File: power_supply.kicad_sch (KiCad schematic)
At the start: 18 parts, among them J1 Разъём к автомобилю 2x16 (32 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, U6 MC78M05CDTG, U7 AMS1117-3.3

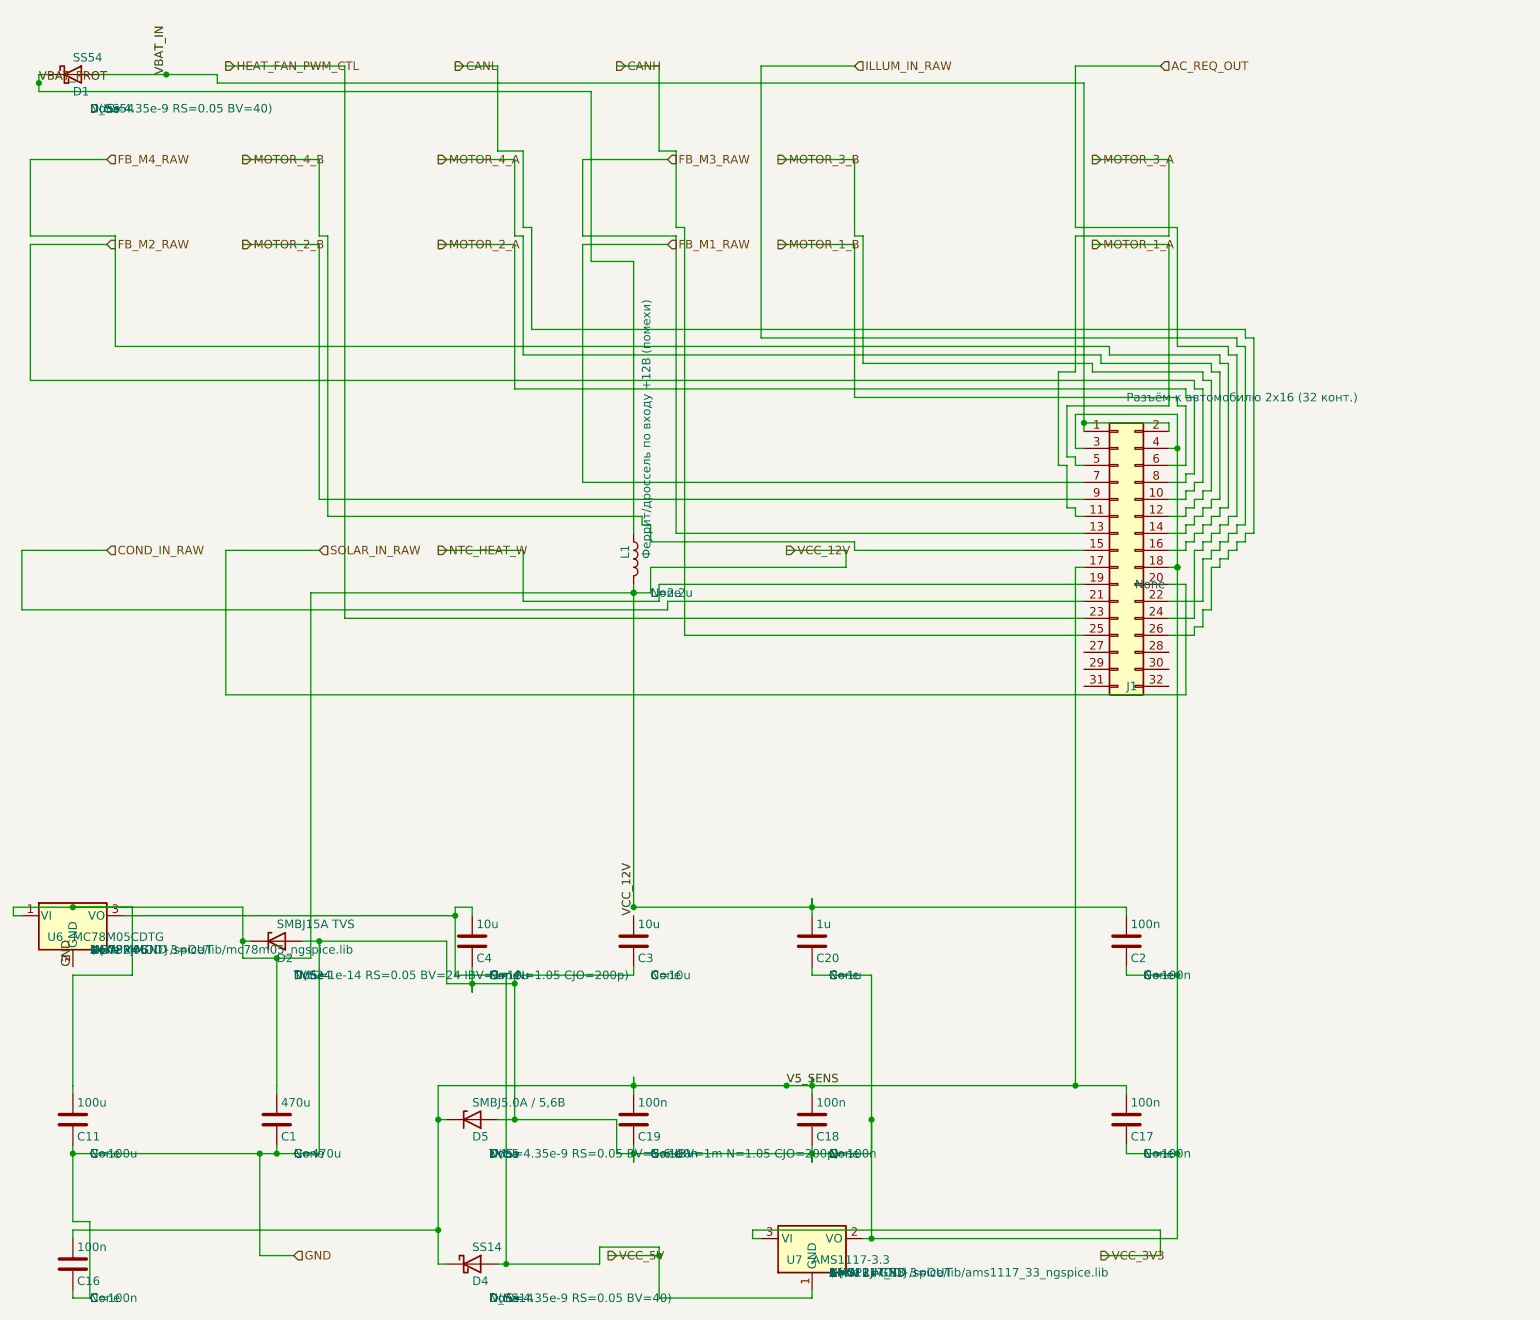
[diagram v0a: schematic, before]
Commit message: multiInstance path fix
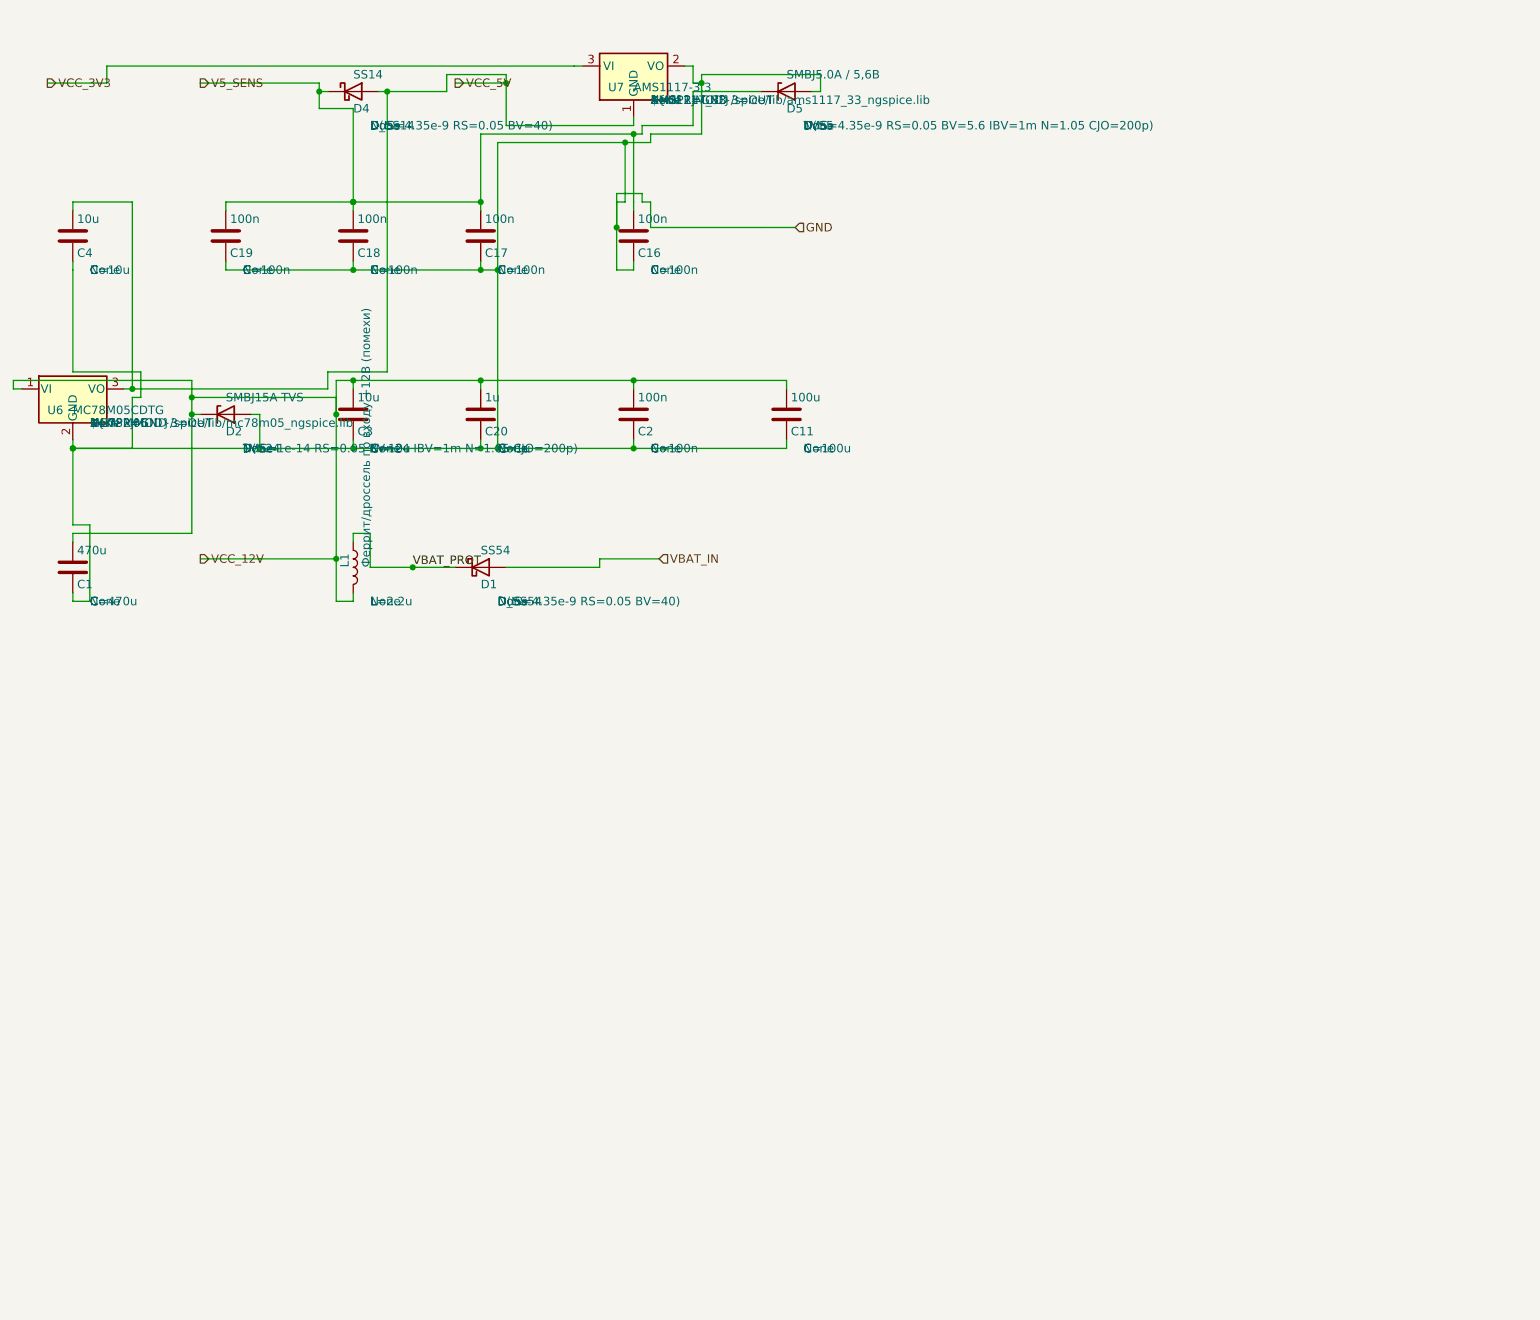
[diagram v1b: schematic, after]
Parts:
- removed J1: Разъём к автомобилю 2x16 (32 конт.), symbol Connector_Generic:Conn_02x16_Odd_Even

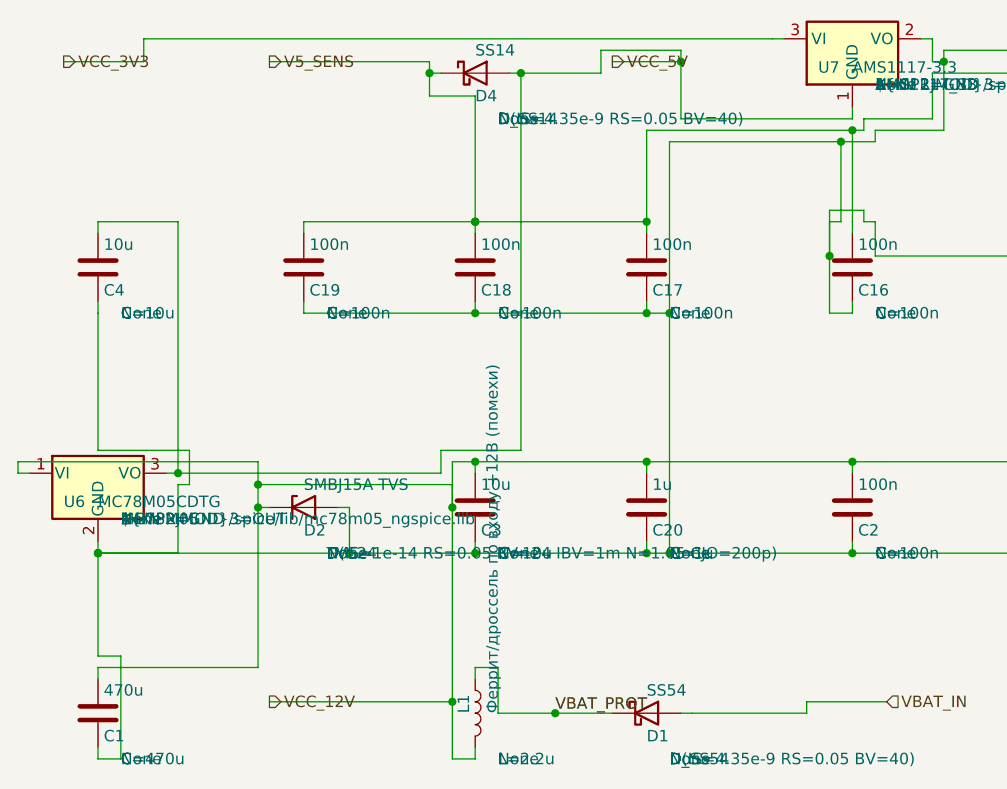
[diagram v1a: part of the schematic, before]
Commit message: fix
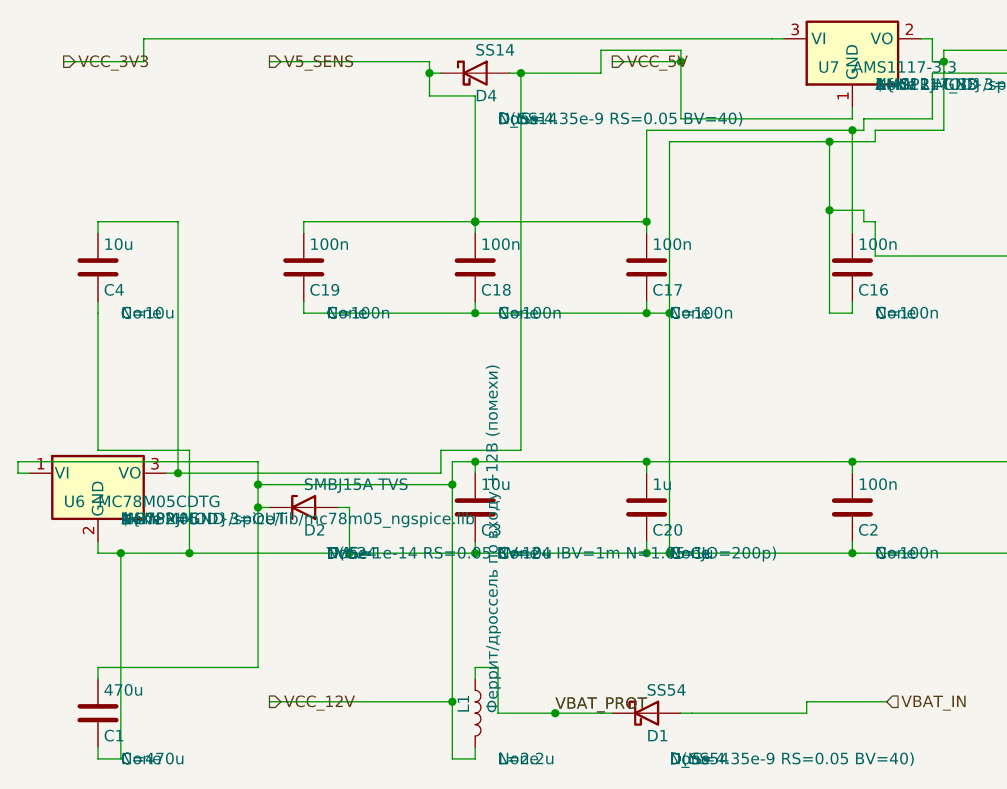
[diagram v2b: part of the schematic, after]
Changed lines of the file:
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@@
 				(instances
 			(project "climate_control_niva_travel"
-				(path "/a20a8d43-2e18-4318-8ef3-7f434a470dab/595b8d41-035e-473d-8fdc-63eaba4c2891"(reference "C0201") (unit 1) )
+				(path "/c1309681-e2dd-46a3-91f6-d828d5f4c0f8"(reference "C1") (unit 1) )
+				(path "/aece091b-8e26-4b21-9786-1b0efc647a51/aaf05096-9cf9-4019-8237-5c0c69cd71a7"(reference "C0201") (unit 1) )
 			)
 		)
@@
 				(instances
 			(project "climate_control_niva_travel"
-				(path "/a20a8d43-2e18-4318-8ef3-7f434a470dab/595b8d41-035e-473d-8fdc-63eaba4c2891"(reference "C0211") (unit 1) )
+				(path "/c1309681-e2dd-46a3-91f6-d828d5f4c0f8"(reference "C11") (unit 1) )
+				(path "/aece091b-8e26-4b21-9786-1b0efc647a51/aaf05096-9cf9-4019-8237-5c0c69cd71a7"(reference "C0211") (unit 1) )
 			)
 		)
@@
 				(instances
 			(project "climate_control_niva_travel"
-				(path "/a20a8d43-2e18-4318-8ef3-7f434a470dab/595b8d41-035e-473d-8fdc-63eaba4c2891"(reference "C0216") (unit 1) )
+				(path "/c1309681-e2dd-46a3-91f6-d828d5f4c0f8"(reference "C16") (unit 1) )
+				(path "/aece091b-8e26-4b21-9786-1b0efc647a51/aaf05096-9cf9-4019-8237-5c0c69cd71a7"(reference "C0216") (unit 1) )
 			)
 		)
@@
 				(instances
 			(project "climate_control_niva_travel"
-				(path "/a20a8d43-2e18-4318-8ef3-7f434a470dab/595b8d41-035e-473d-8fdc-63eaba4c2891"(reference "C0217") (unit 1) )
+				(path "/c1309681-e2dd-46a3-91f6-d828d5f4c0f8"(reference "C17") (unit 1) )
+				(path "/aece091b-8e26-4b21-9786-1b0efc647a51/aaf05096-9cf9-4019-8237-5c0c69cd71a7"(reference "C0217") (unit 1) )
 			)
 		)
@@
 				(instances
 			(project "climate_control_niva_travel"
-				(path "/a20a8d43-2e18-4318-8ef3-7f434a470dab/595b8d41-035e-473d-8fdc-63eaba4c2891"(reference "C0218") (unit 1) )
+				(path "/c1309681-e2dd-46a3-91f6-d828d5f4c0f8"(reference "C18") (unit 1) )
+				(path "/aece091b-8e26-4b21-9786-1b0efc647a51/aaf05096-9cf9-4019-8237-5c0c69cd71a7"(reference "C0218") (unit 1) )
 			)
 		)
@@
 				(instances
 			(project "climate_control_niva_travel"
-				(path "/a20a8d43-2e18-4318-8ef3-7f434a470dab/595b8d41-035e-473d-8fdc-63eaba4c2891"(reference "C0219") (unit 1) )
+				(path "/c1309681-e2dd-46a3-91f6-d828d5f4c0f8"(reference "C19") (unit 1) )
+				(path "/aece091b-8e26-4b21-9786-1b0efc647a51/aaf05096-9cf9-4019-8237-5c0c69cd71a7"(reference "C0219") (unit 1) )
 			)
 		)
@@
 				(instances
 			(project "climate_control_niva_travel"
-				(path "/a20a8d43-2e18-4318-8ef3-7f434a470dab/595b8d41-035e-473d-8fdc-63eaba4c2891"(reference "C0202") (unit 1) )
+				(path "/c1309681-e2dd-46a3-91f6-d828d5f4c0f8"(reference "C2") (unit 1) )
+				(path "/aece091b-8e26-4b21-9786-1b0efc647a51/aaf05096-9cf9-4019-8237-5c0c69cd71a7"(reference "C0202") (unit 1) )
 			)
 		)
@@
 				(instances
 			(project "climate_control_niva_travel"
-				(path "/a20a8d43-2e18-4318-8ef3-7f434a470dab/595b8d41-035e-473d-8fdc-63eaba4c2891"(reference "C0220") (unit 1) )
+				(path "/c1309681-e2dd-46a3-91f6-d828d5f4c0f8"(reference "C20") (unit 1) )
+				(path "/aece091b-8e26-4b21-9786-1b0efc647a51/aaf05096-9cf9-4019-8237-5c0c69cd71a7"(reference "C0220") (unit 1) )
 			)
 		)
@@
 				(instances
 			(project "climate_control_niva_travel"
-				(path "/a20a8d43-2e18-4318-8ef3-7f434a470dab/595b8d41-035e-473d-8fdc-63eaba4c2891"(reference "C0203") (unit 1) )
+				(path "/c1309681-e2dd-46a3-91f6-d828d5f4c0f8"(reference "C3") (unit 1) )
+				(path "/aece091b-8e26-4b21-9786-1b0efc647a51/aaf05096-9cf9-4019-8237-5c0c69cd71a7"(reference "C0203") (unit 1) )
 			)
 		)
@@
 				(instances
 			(project "climate_control_niva_travel"
-				(path "/a20a8d43-2e18-4318-8ef3-7f434a470dab/595b8d41-035e-473d-8fdc-63eaba4c2891"(reference "C0204") (unit 1) )
+				(path "/c1309681-e2dd-46a3-91f6-d828d5f4c0f8"(reference "C4") (unit 1) )
+				(path "/aece091b-8e26-4b21-9786-1b0efc647a51/aaf05096-9cf9-4019-8237-5c0c69cd71a7"(reference "C0204") (unit 1) )
 			)
 		)
@@
 				(instances
 			(project "climate_control_niva_travel"
-				(path "/a20a8d43-2e18-4318-8ef3-7f434a470dab/595b8d41-035e-473d-8fdc-63eaba4c2891"(reference "D0201") (unit 1) )
+				(path "/c1309681-e2dd-46a3-91f6-d828d5f4c0f8"(reference "D1") (unit 1) )
+				(path "/aece091b-8e26-4b21-9786-1b0efc647a51/aaf05096-9cf9-4019-8237-5c0c69cd71a7"(reference "D0201") (unit 1) )
 			)
 		)
@@
 				(instances
 			(project "climate_control_niva_travel"
-				(path "/a20a8d43-2e18-4318-8ef3-7f434a470dab/595b8d41-035e-473d-8fdc-63eaba4c2891"(reference "D0202") (unit 1) )
+				(path "/c1309681-e2dd-46a3-91f6-d828d5f4c0f8"(reference "D2") (unit 1) )
+				(path "/aece091b-8e26-4b21-9786-1b0efc647a51/aaf05096-9cf9-4019-8237-5c0c69cd71a7"(reference "D0202") (unit 1) )
 			)
 		)
@@
 				(instances
 			(project "climate_control_niva_travel"
-				(path "/a20a8d43-2e18-4318-8ef3-7f434a470dab/595b8d41-035e-473d-8fdc-63eaba4c2891"(reference "D0204") (unit 1) )
+				(path "/c1309681-e2dd-46a3-91f6-d828d5f4c0f8"(reference "D4") (unit 1) )
+				(path "/aece091b-8e26-4b21-9786-1b0efc647a51/aaf05096-9cf9-4019-8237-5c0c69cd71a7"(reference "D0204") (unit 1) )
 			)
 		)
@@
 				(instances
 			(project "climate_control_niva_travel"
-				(path "/a20a8d43-2e18-4318-8ef3-7f434a470dab/595b8d41-035e-473d-8fdc-63eaba4c2891"(reference "D0205") (unit 1) )
+				(path "/c1309681-e2dd-46a3-91f6-d828d5f4c0f8"(reference "D5") (unit 1) )
+				(path "/aece091b-8e26-4b21-9786-1b0efc647a51/aaf05096-9cf9-4019-8237-5c0c69cd71a7"(reference "D0205") (unit 1) )
 			)
 		)
@@
 				(instances
 			(project "climate_control_niva_travel"
-				(path "/a20a8d43-2e18-4318-8ef3-7f434a470dab/595b8d41-035e-473d-8fdc-63eaba4c2891"(reference "L0201") (unit 1) )
+				(path "/c1309681-e2dd-46a3-91f6-d828d5f4c0f8"(reference "L1") (unit 1) )
+				(path "/aece091b-8e26-4b21-9786-1b0efc647a51/aaf05096-9cf9-4019-8237-5c0c69cd71a7"(reference "L0201") (unit 1) )
 			)
 		)
@@
 				(instances
 			(project "climate_control_niva_travel"
-				(path "/a20a8d43-2e18-4318-8ef3-7f434a470dab/595b8d41-035e-473d-8fdc-63eaba4c2891"(reference "U0206") (unit 1) )
+				(path "/c1309681-e2dd-46a3-91f6-d828d5f4c0f8"(reference "U6") (unit 1) )
+				(path "/aece091b-8e26-4b21-9786-1b0efc647a51/aaf05096-9cf9-4019-8237-5c0c69cd71a7"(reference "U0206") (unit 1) )
 			)
 		)
@@
 				(instances
 			(project "climate_control_niva_travel"
-				(path "/a20a8d43-2e18-4318-8ef3-7f434a470dab/595b8d41-035e-473d-8fdc-63eaba4c2891"(reference "U0207") (unit 1) )
+				(path "/c1309681-e2dd-46a3-91f6-d828d5f4c0f8"(reference "U7") (unit 1) )
+				(path "/aece091b-8e26-4b21-9786-1b0efc647a51/aaf05096-9cf9-4019-8237-5c0c69cd71a7"(reference "U0207") (unit 1) )
 			)
 		)
@@
 	(wire
 		(pts
-			(xy 50.8 53.34) (xy 50.8 55.88)
-		)
-		(stroke
-			(width 0)
-			(type default)
-		)
-	)
-	(wire
-		(pts
 			(xy 11.43 74.93) (xy 11.43 73.66)
 		)
@@
 	(wire
 		(pts
-			(xy 13.97 83.82) (xy 13.97 72.39)
-		)
-		(stroke
-			(width 0)
-			(type default)
-		)
-	)
-	(wire
-		(pts
-			(xy 13.97 72.39) (xy 11.43 72.39)
-		)
-		(stroke
-			(width 0)
-			(type default)
-		)
-	)
-	(wire
-		(pts
-			(xy 11.43 72.39) (xy 11.43 60.96)
+			(xy 13.97 83.82) (xy 13.97 60.96)
 		)
 		(stroke
@@
 	(wire
 		(pts
-			(xy 21.59 49.53) (xy 21.59 53.34)
-		)
-		(stroke
-			(width 0)
-			(type default)
-		)
-	)
-	(wire
-		(pts
-			(xy 21.59 53.34) (xy 20.32 53.34)
-		)
-		(stroke
-			(width 0)
-			(type default)
-		)
-	)
-	(wire
-		(pts
-			(xy 20.32 53.34) (xy 20.32 60.96)
-		)
-		(stroke
-			(width 0)
-			(type default)
-		)
-	)
-	(wire
-		(pts
-			(xy 20.32 60.96) (xy 11.43 60.96)
+			(xy 21.59 49.53) (xy 21.59 60.96)
 		)
 		(stroke
@@
 	(wire
 		(pts
-			(xy 92.71 34.29) (xy 92.71 24.13)
-		)
-		(stroke
-			(width 0)
-			(type default)
-		)
-	)
-	(wire
-		(pts
-			(xy 92.71 24.13) (xy 93.98 24.13)
-		)
-		(stroke
-			(width 0)
-			(type default)
-		)
-	)
-	(wire
-		(pts
-			(xy 93.98 24.13) (xy 93.98 15.24)
+			(xy 92.71 34.29) (xy 92.71 15.24)
 		)
 		(stroke
@@
 		)
 	)
-	(wire
-		(pts
-			(xy 92.71 22.86) (xy 92.71 27.94)
-		)
-		(stroke
-			(width 0)
-			(type default)
-		)
-	)
 	(junction
 		(at 53.34 50.8)
@@
 	)
 	(junction
-		(at 50.8 55.88)
+		(at 50.8 53.34)
 		(diameter 0.0000)
 		(color 0 0 0 0)
@@
 	)
 	(junction
-		(at 11.43 60.96)
+		(at 13.97 60.96)
 		(diameter 0.0000)
 		(color 0 0 0 0)
@@
 	)
 	(junction
-		(at 11.43 60.96)
+		(at 21.59 60.96)
 		(diameter 0.0000)
 		(color 0 0 0 0)
@@
 	)
 	(junction
-		(at 93.98 15.24)
+		(at 92.71 15.24)
 		(diameter 0.0000)
 		(color 0 0 0 0)
@@
 	)
 	(junction
-		(at 92.71 27.94)
-		(diameter 0.0000)
-		(color 0 0 0 0)
+		(at 92.71 22.86)
+		(diameter 0.0000)
+		(color 0 0 0 0)
